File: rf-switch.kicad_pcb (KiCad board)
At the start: 2 copper layers, 60.2 x 36.4 mm, 14 parts, among them IC1 PE42440MLBB-Z, J1 Conn_01x04_Pin, J2 Conn_Coaxial_Small, J3 Conn_Coaxial_Small, J4 Conn_Coaxial_Small, J5 Conn_Coaxial_Small, J6 Conn_Coaxial_Small

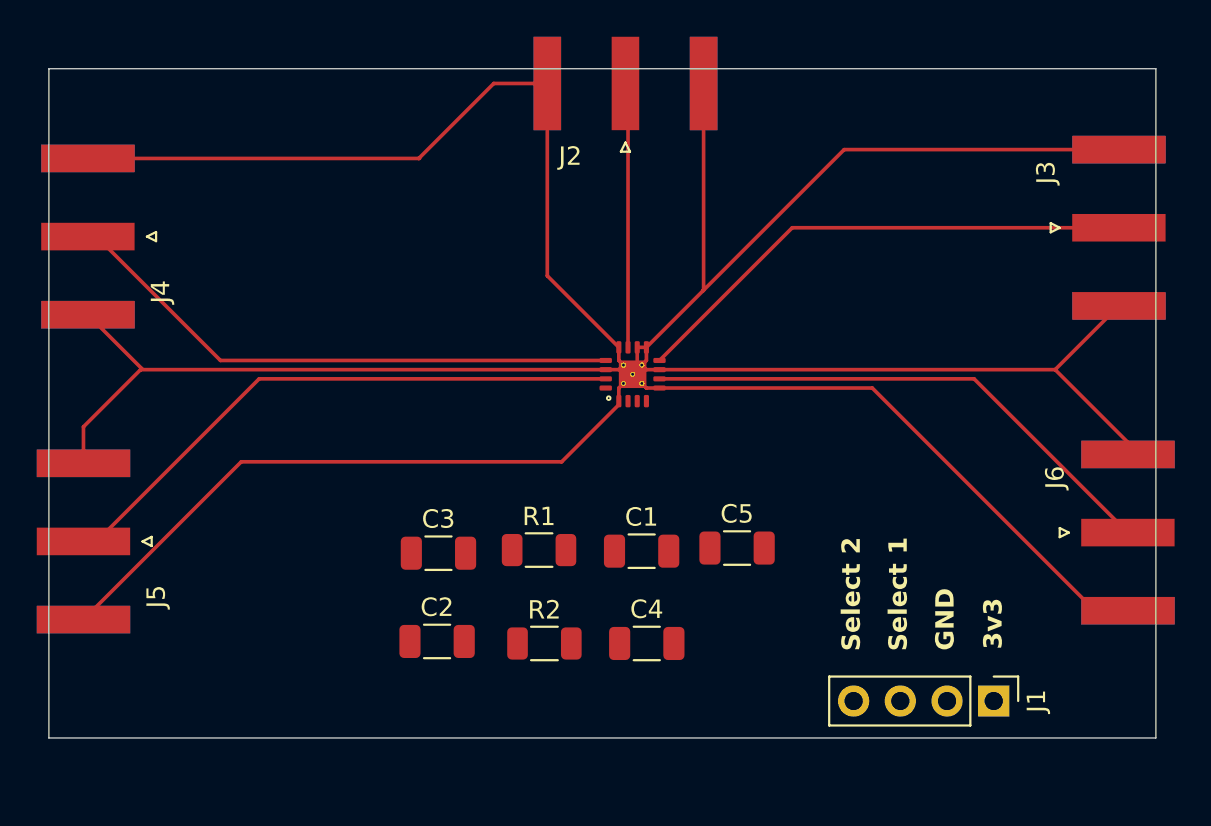
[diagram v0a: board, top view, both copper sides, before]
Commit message: PCB layout is done
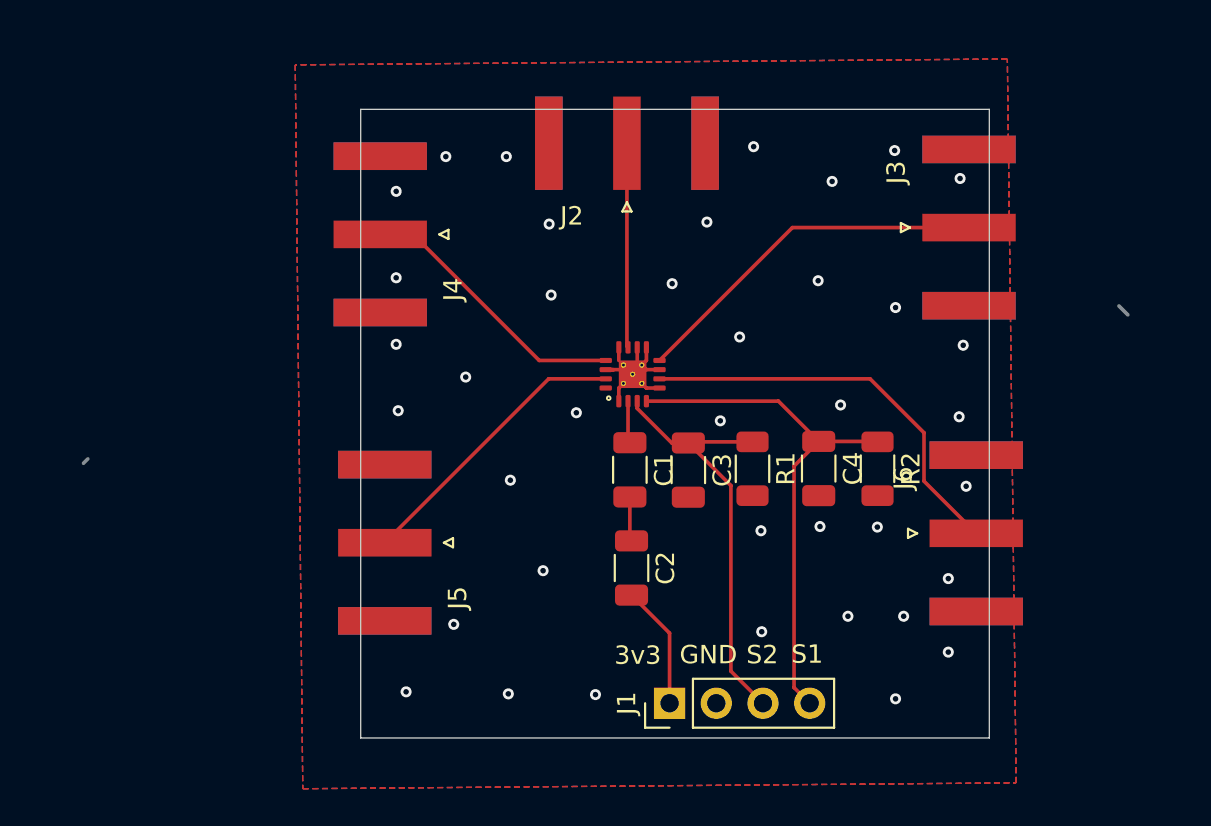
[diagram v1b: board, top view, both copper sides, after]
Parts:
- removed C5: 0.01u, Capacitor_SMD:C_1206_3216Metric
- C2: value 0.01u -> 10u
- C3: value 10u -> 0.01u
- R1, R2: value 1M -> 10k
- moved R2 20.5 mm to (169.4, 101.5), turned to -90 degrees
- moved J1 17.6 mm to (158.1, 114.3), turned to 90 degrees
- moved J5 16.4 mm to (142.6, 105.5)
- moved J4 15.9 mm to (142.3, 88.8)
- moved C3 14.3 mm to (159.1, 101.6), turned to -90 degrees
- moved C4 13.3 mm to (166.2, 101.5), turned to -90 degrees
- moved R1 12.4 mm to (162.6, 101.5), turned to -90 degrees
- moved C2 11.3 mm to (156.0, 106.9), turned to -90 degrees
- moved J6 8.25 mm to (174.8, 105.0)
- moved J3 8.15 mm to (174.4, 88.4)
- moved C1 4.47 mm to (155.9, 101.6), turned to -90 degrees
- moved J2 3.25 mm to (155.8, 83.8)
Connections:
- C1 pad 1: /Select_2 -> Net-(IC1-VDD)
- C1 pad 2: GND -> Net-(C1-Pad2)
- C2 pad 1: /Select_1 -> Net-(C1-Pad2)
- C2 pad 2: GND -> /3v3
- C3 pad 1: Net-(C3-Pad1) -> /Select_2
- C4 pad 1: GND -> /Select_1
- IC1 pad 2: /3v3 -> Net-(IC1-VDD)
- R1 pad 1: Net-(C3-Pad1) -> /Select_2
- R1 pad 2: /Select_2 -> GND
- R2 pad 1: Net-(C3-Pad1) -> /Select_1
- R2 pad 2: /Select_1 -> GND
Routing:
- net GND: track 226.9 -> 11.2 mm, vias 0 -> 39
- net /Select_1: track 0.00 -> 29.3 mm
- net /Select_2: track 0.00 -> 23.3 mm
- net Net-(IC1-RF2): track 31.4 -> 15.7 mm
- net Net-(IC1-RF1): track 30.5 -> 15.1 mm
- net Net-(IC1-RF3): track 28.0 -> 19.8 mm
- net /3v3: track 0.00 -> 6.74 mm
- net Net-(IC1-RF4): track 28.9 -> 22.2 mm
- net Net-(IC1-RFC): track 14.4 -> 11.1 mm
- net Net-(C1-Pad2): track 0.00 -> 2.43 mm
- net Net-(IC1-VDD): track 0.00 -> 2.30 mm
- added copper zone on B.Cu, net GND
- added copper zone on F.Cu, net GND
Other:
- board size 60.2 x 36.4 mm -> 34.2 x 34.2 mm
- board text added: "S1"
- board text added: "S2"
- board text removed: "Select 1"
- board text removed: "Select 2"
